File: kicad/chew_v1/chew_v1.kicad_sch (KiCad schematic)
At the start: 19 parts, among them U1 RP2040_Zero, U2 TRRS

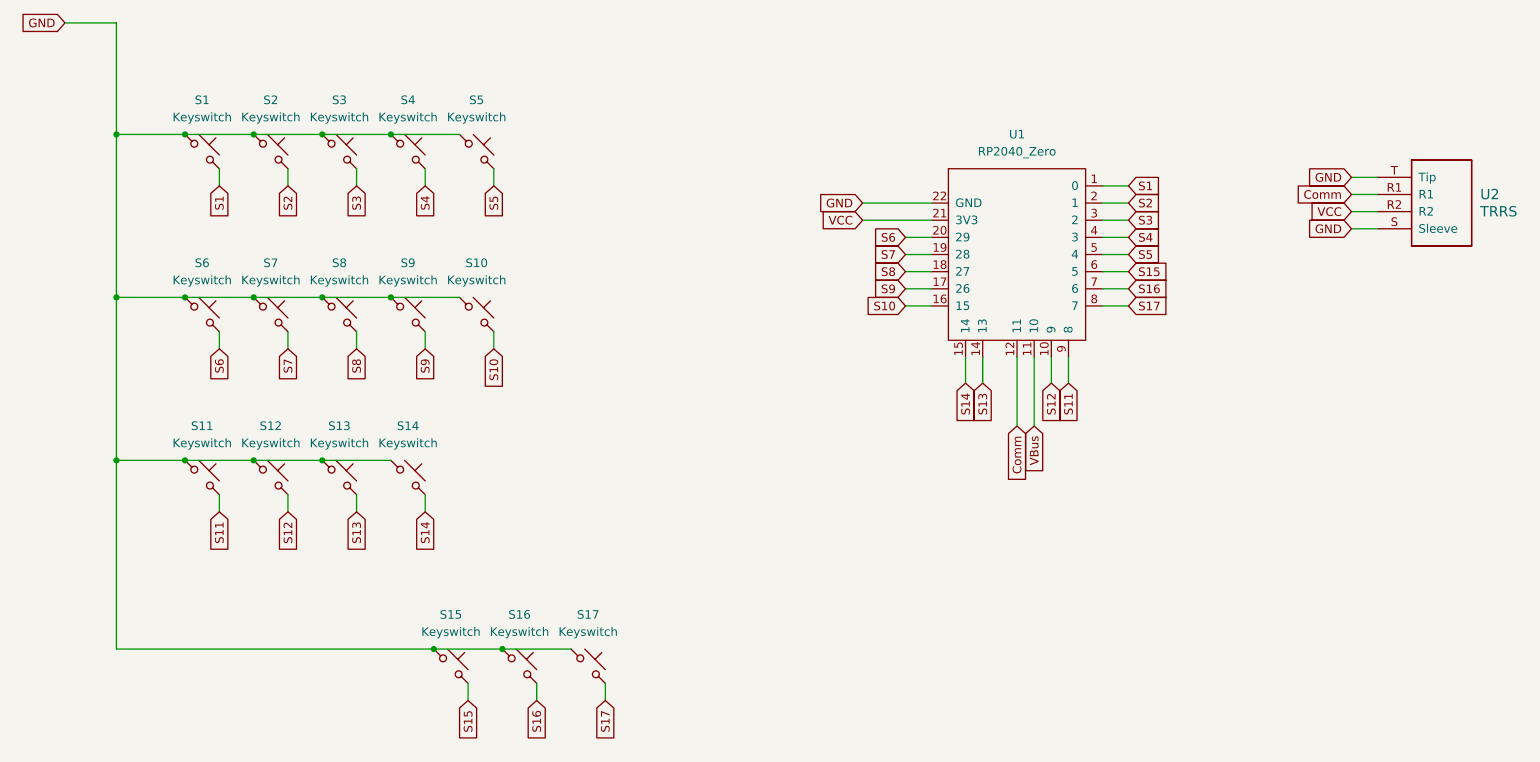
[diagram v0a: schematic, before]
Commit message: Replace footprints
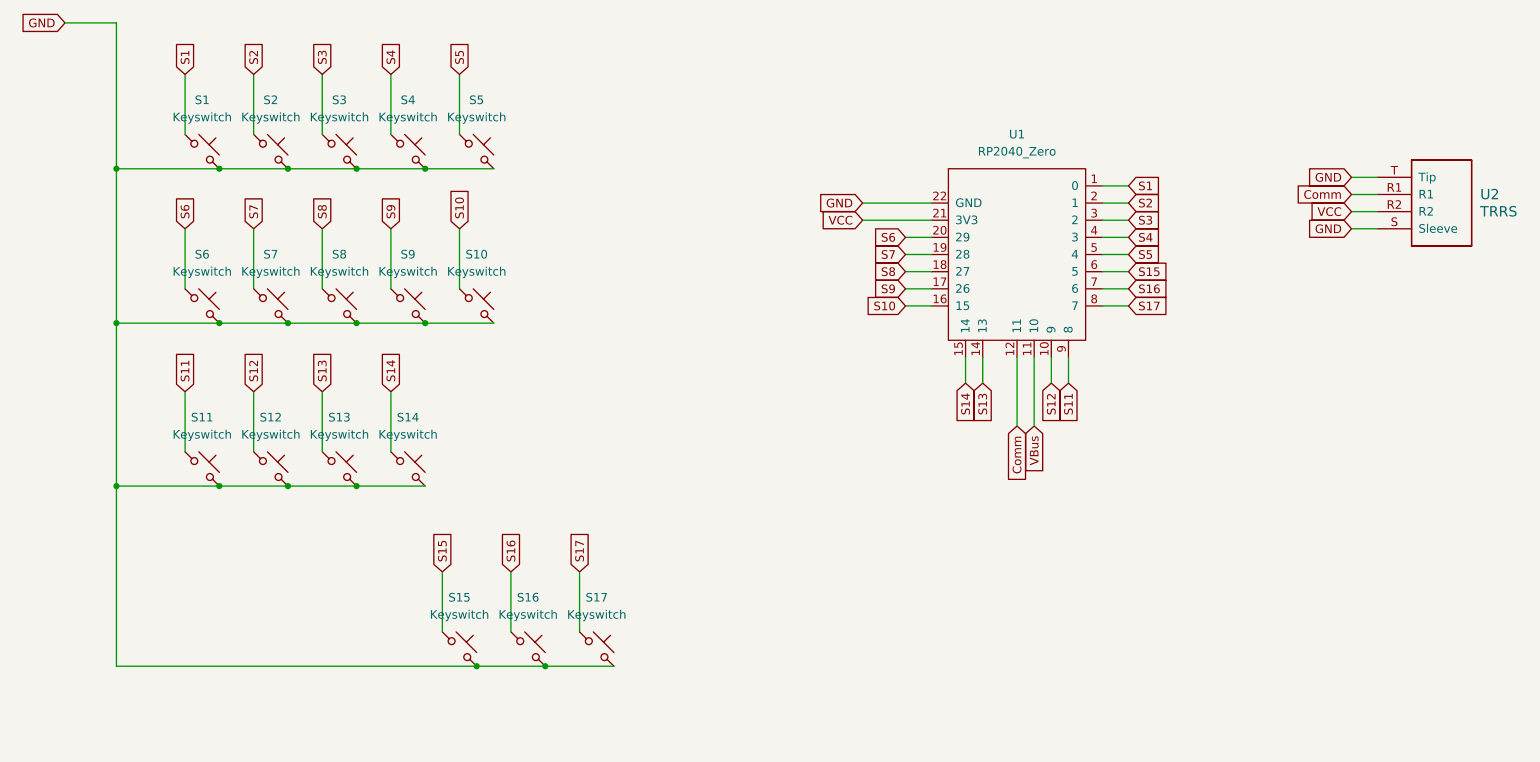
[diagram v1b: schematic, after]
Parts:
- S1, S11, S12, S14, S16, S17, S3, S5, S7, S8, S9: symbol ScottoKeebs:Placeholder_Keyswitch -> chew_symbols:Placeholder_Keyswitch
- S10, S13, S15, S2, S4, S6: footprint chew_is_so:Choc_V1_chew_reversible_1 -> chew_is_so:Choc_V1_chew_reversible_2; symbol ScottoKeebs:Placeholder_Keyswitch -> chew_symbols:Placeholder_Keyswitch
- U1: symbol ScottoKeebs:MCU_RP2040_Zero -> chew_symbols:MCU_RP2040_Zero_reversible
- U2: symbol ScottoKeebs:Placeholder_TRRS -> chew_symbols:Placeholder_TRRS
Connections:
- net GND: now also S1.2, S10.2, S11.2, S12.2, S13.2, S14.2, S15.2, S16.2, S17.2, S2.2, S3.2, S4.2, S5.2, S6.2, S7.2, S8.2, S9.2; no longer S1.1, S10.1, S11.1, S12.1, S13.1, S14.1, S15.1, S16.1, S17.1, S2.1, S3.1, S4.1, S5.1, S6.1, S7.1, S8.1, S9.1
- net S1: now also S1.1; no longer S1.2
- net S10: now also S10.1; no longer S10.2
- net S11: now also S11.1; no longer S11.2
- net S12: now also S12.1; no longer S12.2
- net S13: now also S13.1; no longer S13.2
- net S14: now also S14.1; no longer S14.2
- net S15: now also S15.1; no longer S15.2
- net S16: now also S16.1; no longer S16.2
- net S17: now also S17.1; no longer S17.2
- net S2: now also S2.1; no longer S2.2
- net S3: now also S3.1; no longer S3.2
- net S4: now also S4.1; no longer S4.2
- net S5: now also S5.1; no longer S5.2
- net S6: now also S6.1; no longer S6.2
- net S7: now also S7.1; no longer S7.2
- net S8: now also S8.1; no longer S8.2
- net S9: now also S9.1; no longer S9.2
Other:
- moved on the sheet: S10, S11, S12, S13, S14, S15, S16, S17, S6, S7, S8, S9
